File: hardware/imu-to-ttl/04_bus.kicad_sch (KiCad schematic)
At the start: 12 parts, among them U3 SN74LVC2G241DCUR

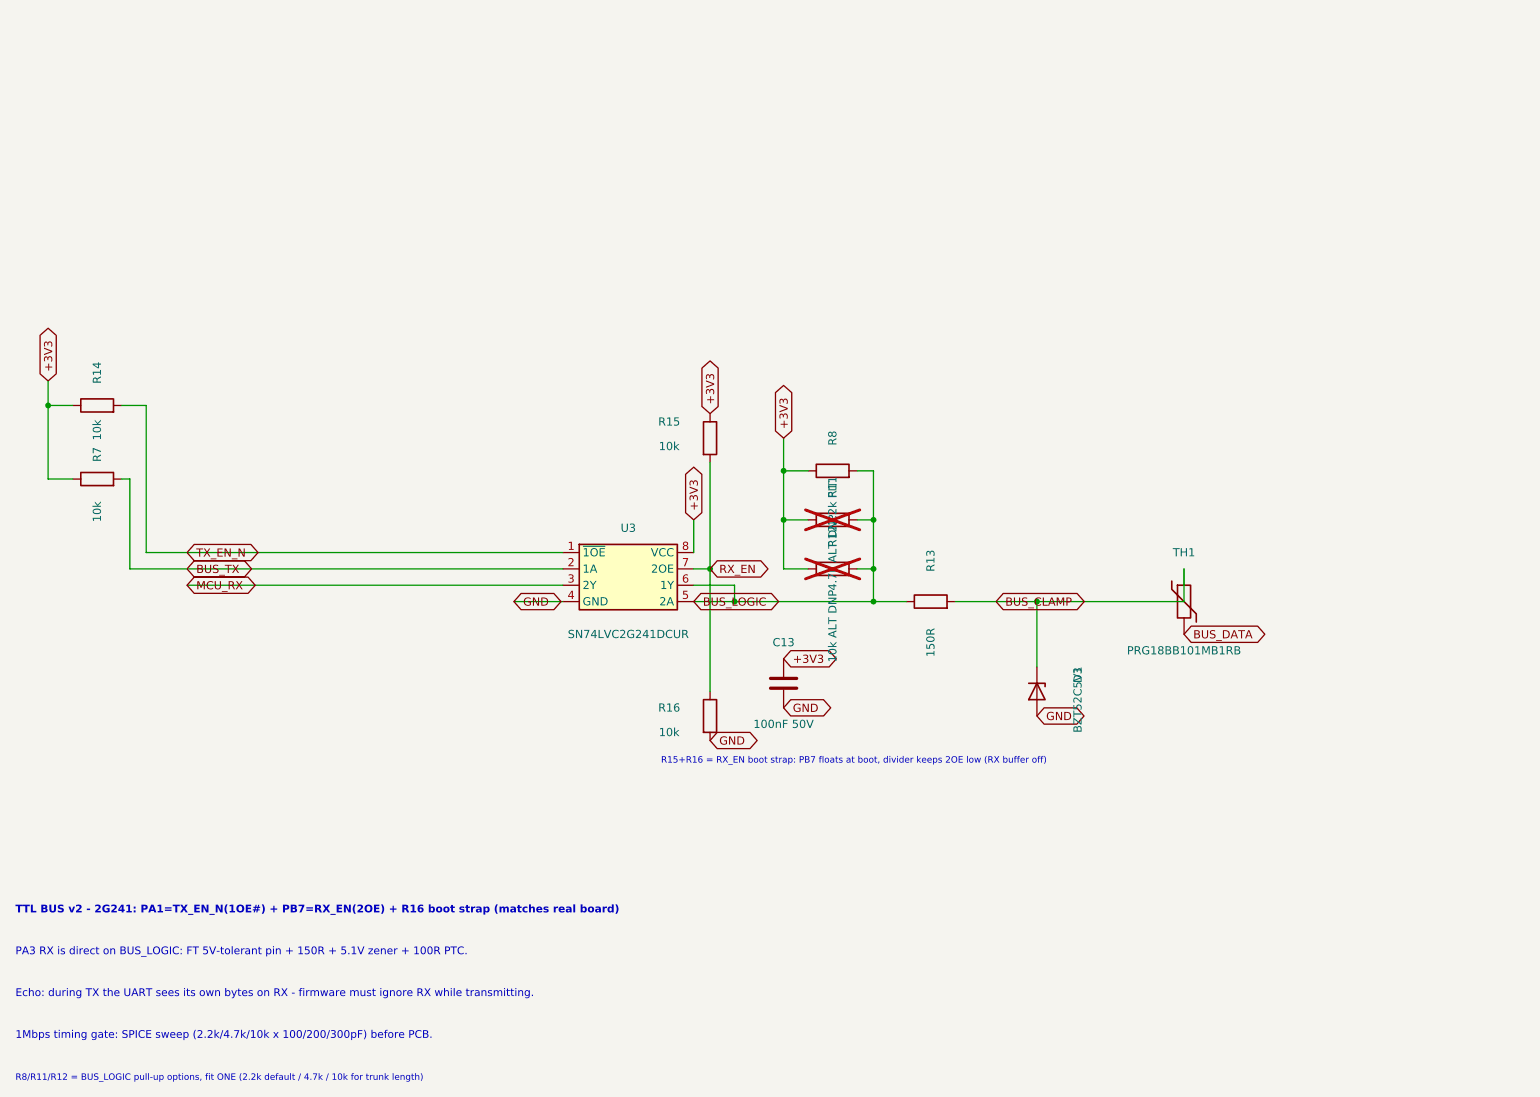
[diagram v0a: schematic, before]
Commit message: sync: 2026-10-15 日常更新
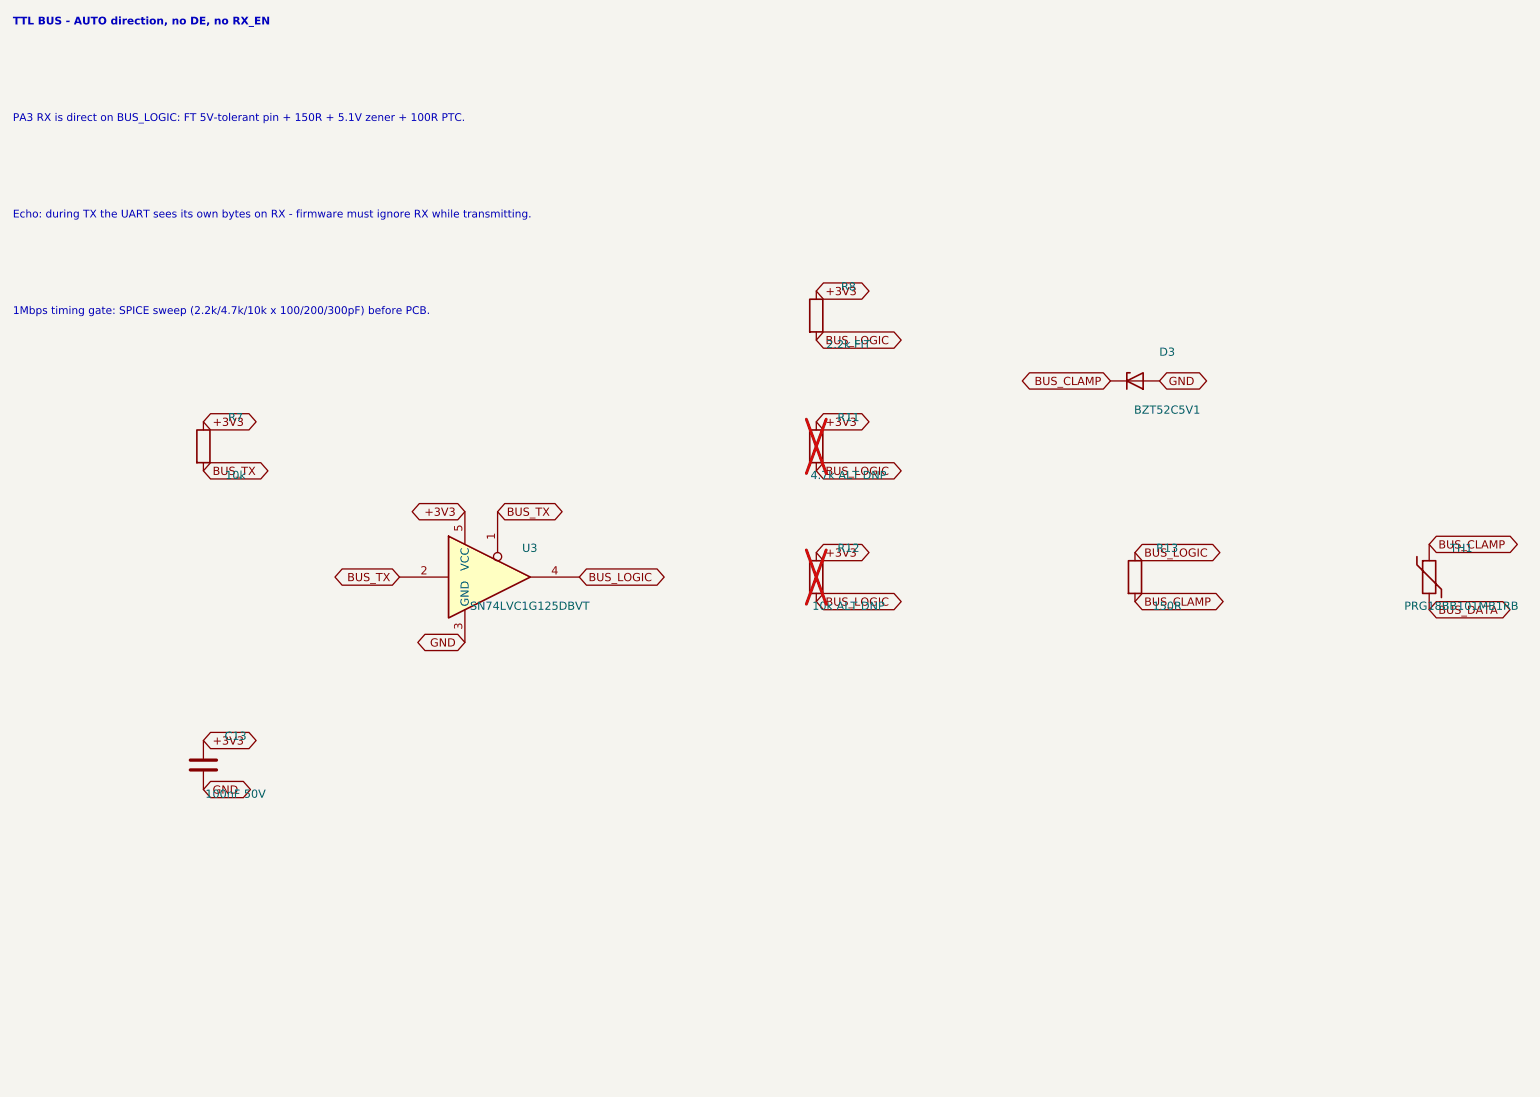
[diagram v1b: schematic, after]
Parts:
- removed R14, R15, R16: 10k, Resistor_SMD:R_0603_1608Metric, symbol Device:R
- removed U3: SN74LVC2G241DCUR, Package_SO:TSSOP-8_3x3mm_P0.65mm, symbol 74xGxx:SN74LVC2G241
- added U3: SN74LVC1G125DBVT, Package_TO_SOT_SMD:SOT-23-5, symbol 74xGxx:74LVC1G125
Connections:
- net +3V3: now also U3.5 (VCC)
- net BUS_LOGIC: now also U3.4
- net BUS_TX: now also U3.1, U3.2
- net GND: now also U3.3 (GND)
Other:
- note added: "TTL BUS - AUTO direction, no DE, no RX_EN"
- note removed: "R15+R16 = RX_EN boot strap: PB7 floats at boot, divider keeps 2OE low (RX buffer off)"
- note removed: "R8/R11/R12 = BUS_LOGIC pull-up options, fit ONE (2.2k default / 4.7k / 10k for trunk length)"
- note removed: "TTL BUS v2 - 2G241: PA1=TX_EN_N(1OE#) + PB7=RX_EN(2OE) + R16 boot strap (matches real board)"

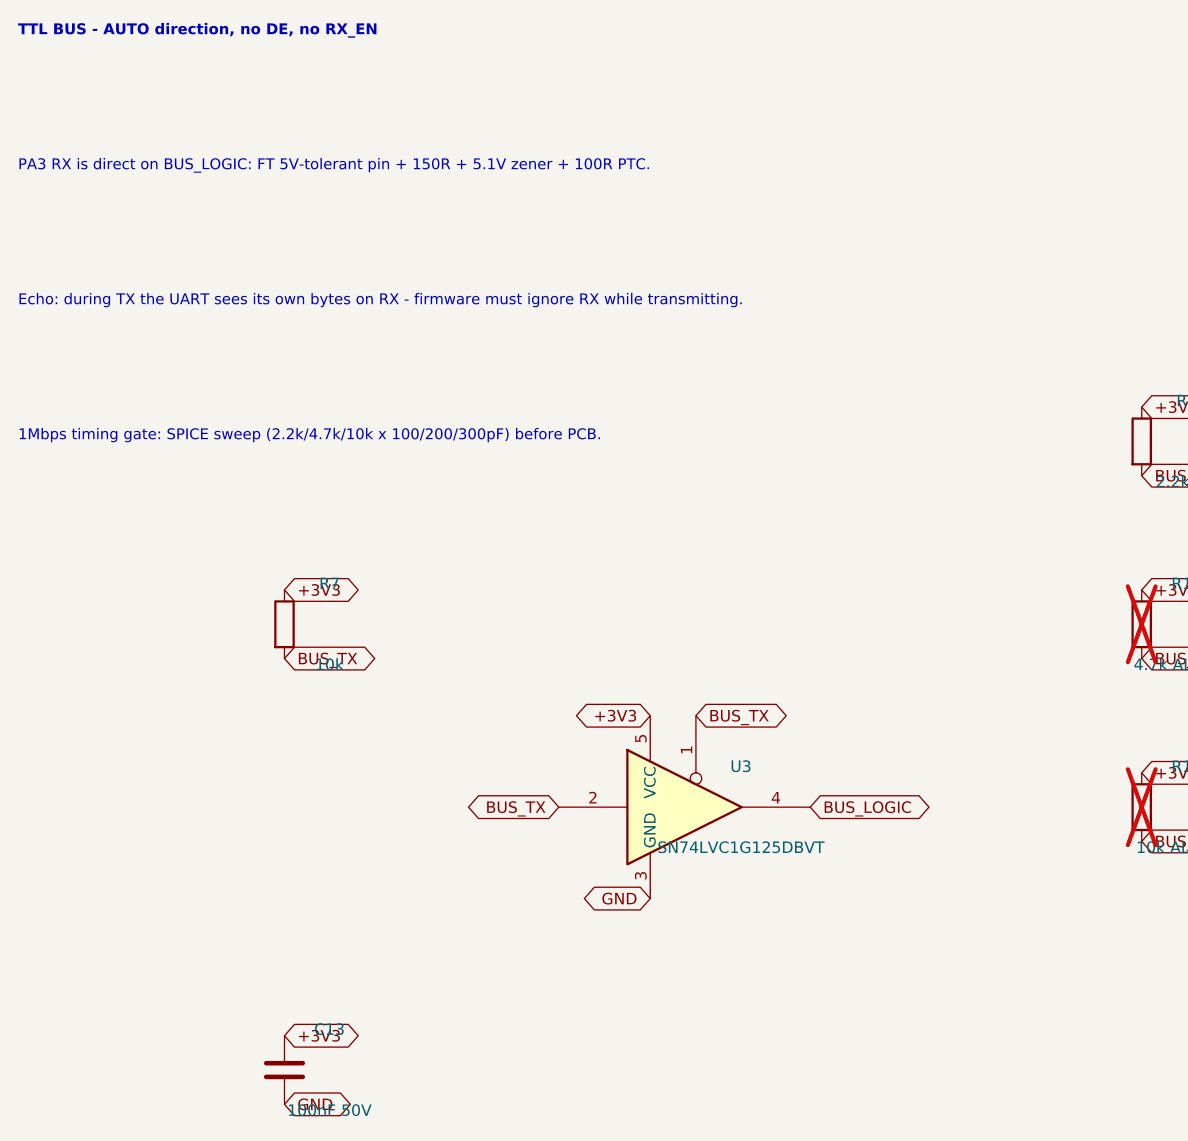
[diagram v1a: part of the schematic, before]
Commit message: sync: 2026-10-12 日常更新
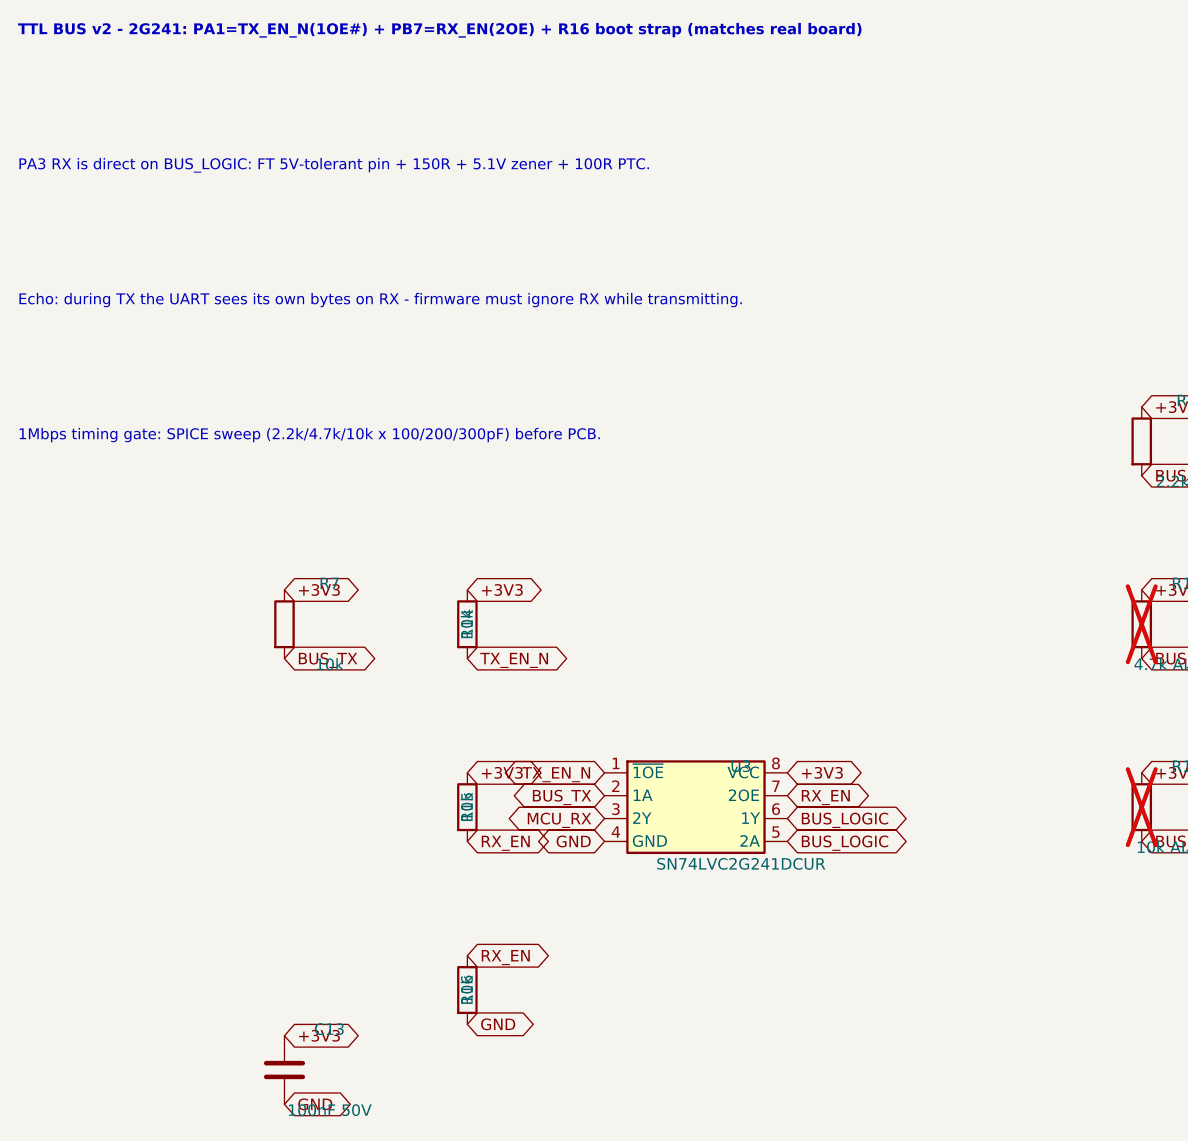
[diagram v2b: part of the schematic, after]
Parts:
- removed U3: SN74LVC1G125DBVT, Package_TO_SOT_SMD:SOT-23-5, symbol 74xGxx:74LVC1G125
- added R14, R15, R16: 10k, Resistor_SMD:R_0603_1608Metric, symbol Device:R
- added U3: SN74LVC2G241DCUR, Package_SO:TSSOP-8_3x3mm_P0.65mm, symbol 74xGxx:SN74LVC2G241
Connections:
- net +3V3: now also R14.1, R15.1, U3.8 (VCC)
- net BUS_LOGIC: now also U3.5 (2A), U3.6 (1Y)
- net BUS_TX: now also U3.2 (1A)
- net GND: now also R16.2, U3.4 (GND)
- new net MCU_RX: U3.3 (2Y)
- new net RX_EN: R15.2, R16.1, U3.7 (2OE)
- new net TX_EN_N: R14.2, U3.1 (~{1OE})
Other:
- note added: "TTL BUS v2 - 2G241: PA1=TX_EN_N(1OE#) + PB7=RX_EN(2OE) + R16 boot strap (matches real board)"
- note removed: "TTL BUS - AUTO direction, no DE, no RX_EN"

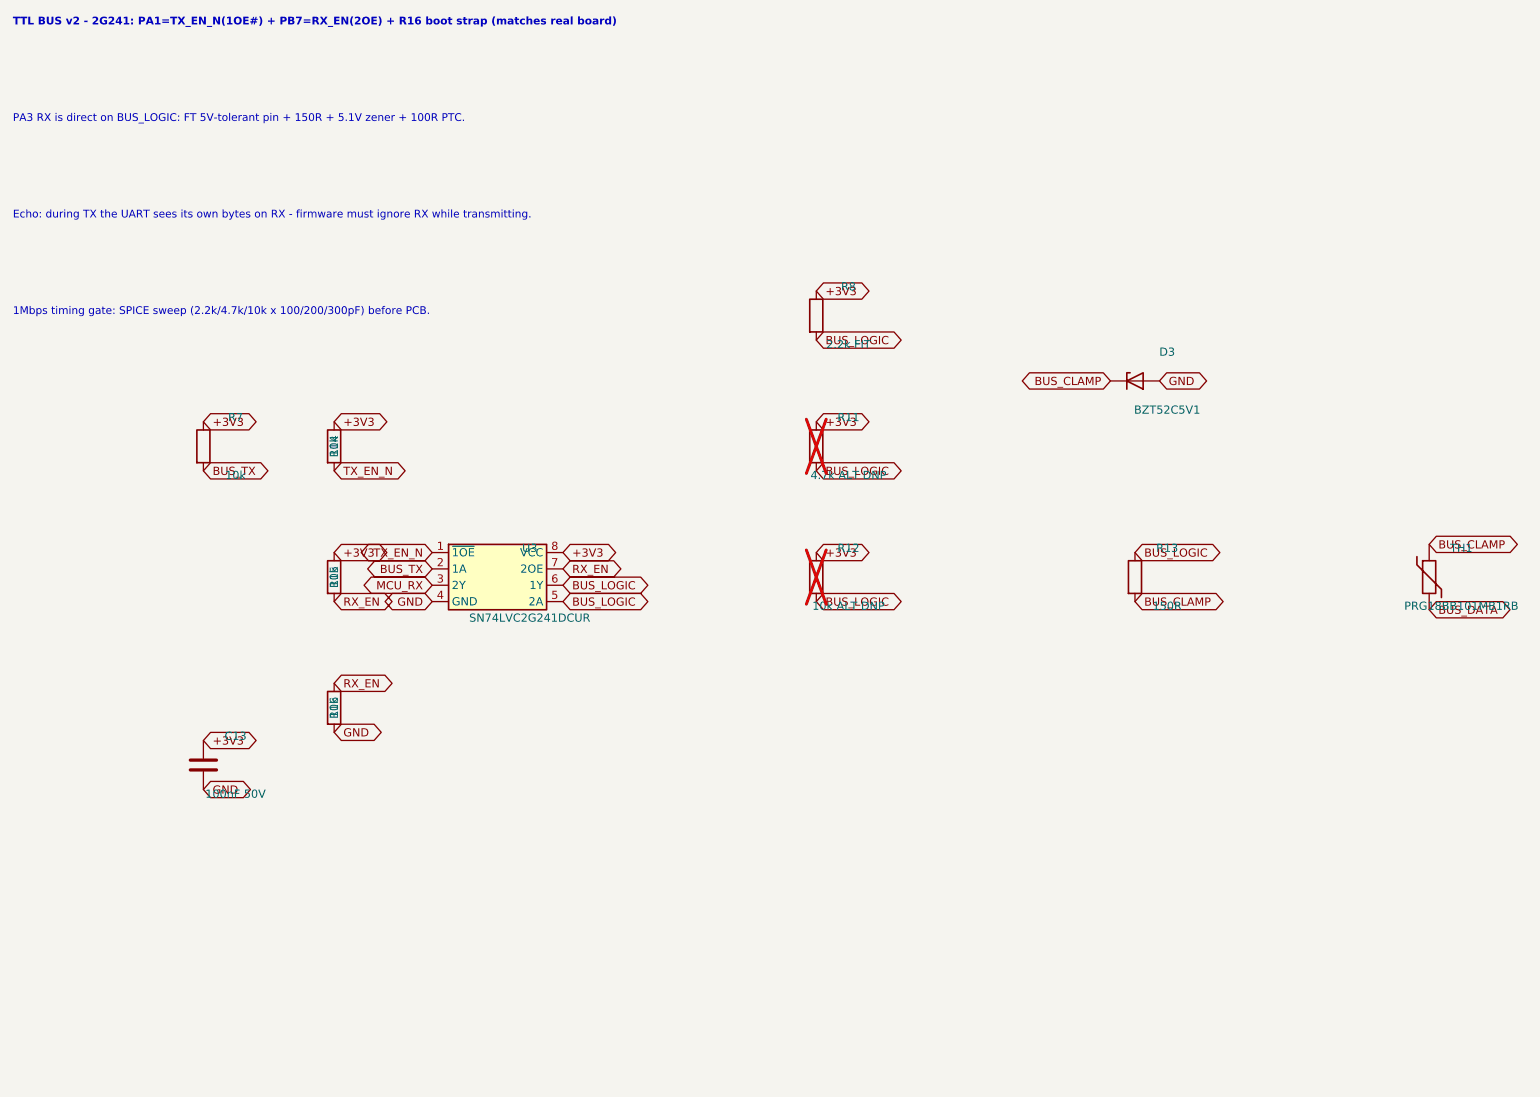
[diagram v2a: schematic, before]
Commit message: sync: 2026-10-12 日常更新
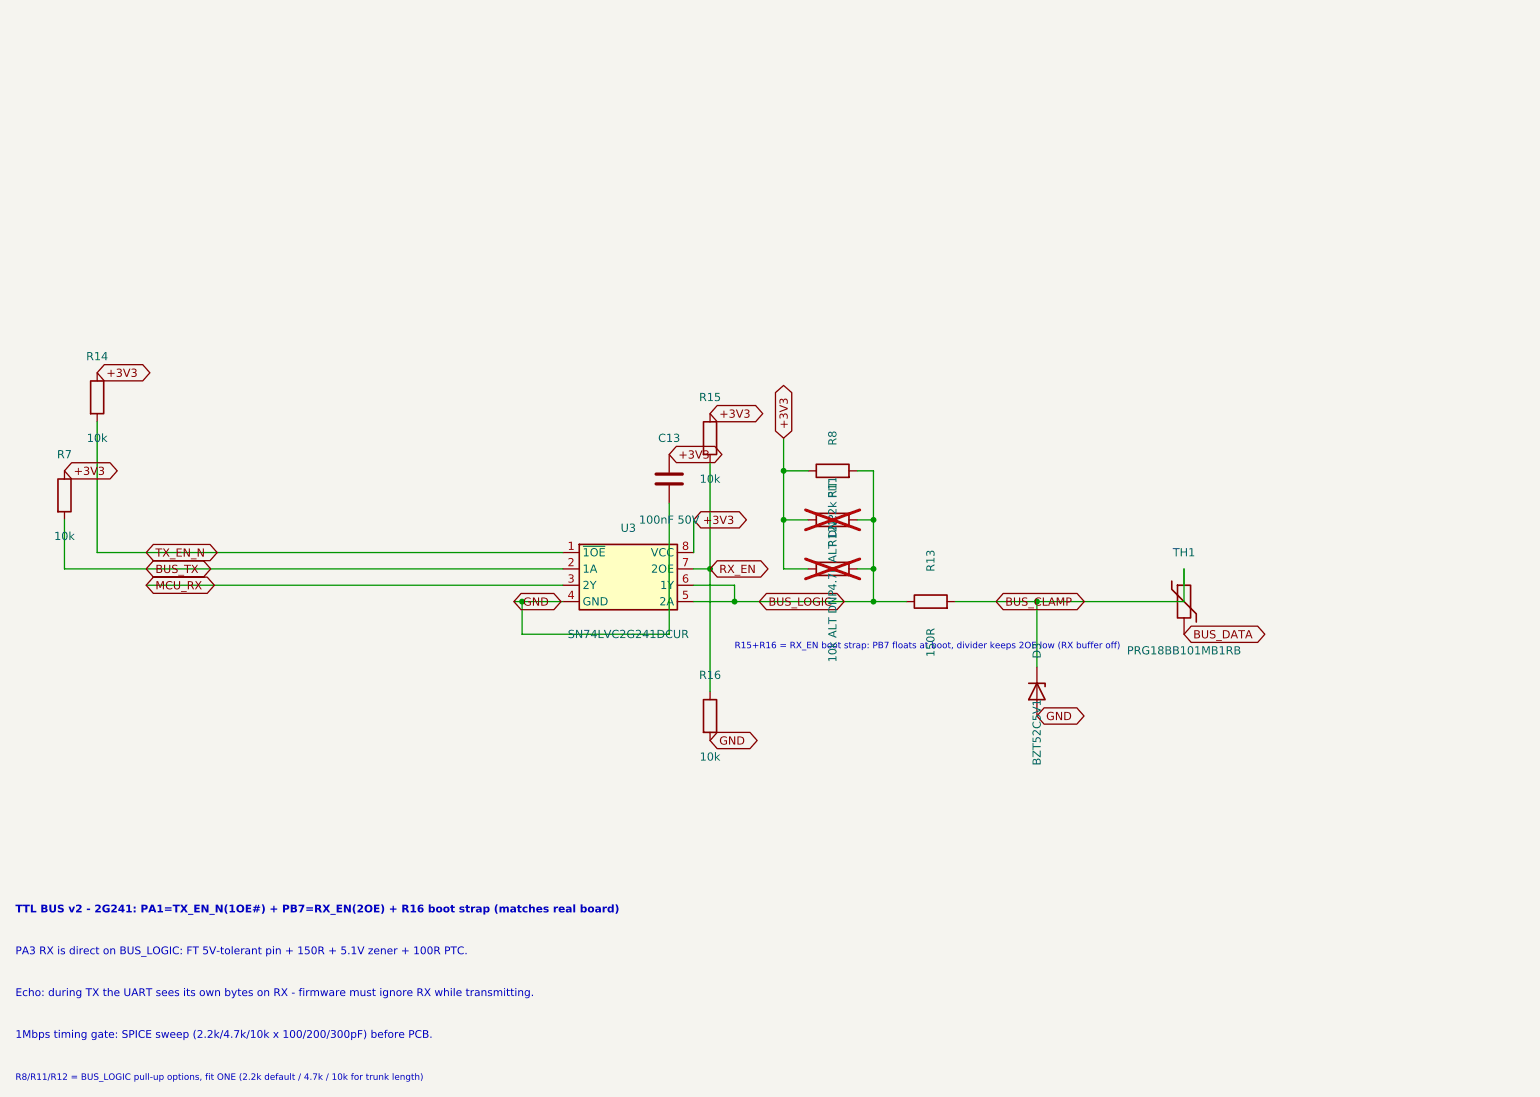
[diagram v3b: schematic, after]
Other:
- note added: "R15+R16 = RX_EN boot strap: PB7 floats at boot, divider keeps 2OE low (RX buffer off)"
- note added: "R8/R11/R12 = BUS_LOGIC pull-up options, fit ONE (2.2k default / 4.7k / 10k for trunk length)"
